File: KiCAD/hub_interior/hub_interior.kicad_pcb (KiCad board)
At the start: 2 copper layers, 50 x 50 mm, 15 parts, among them Q1 BC337, X2 BUZZER, X3 LED_ROJO

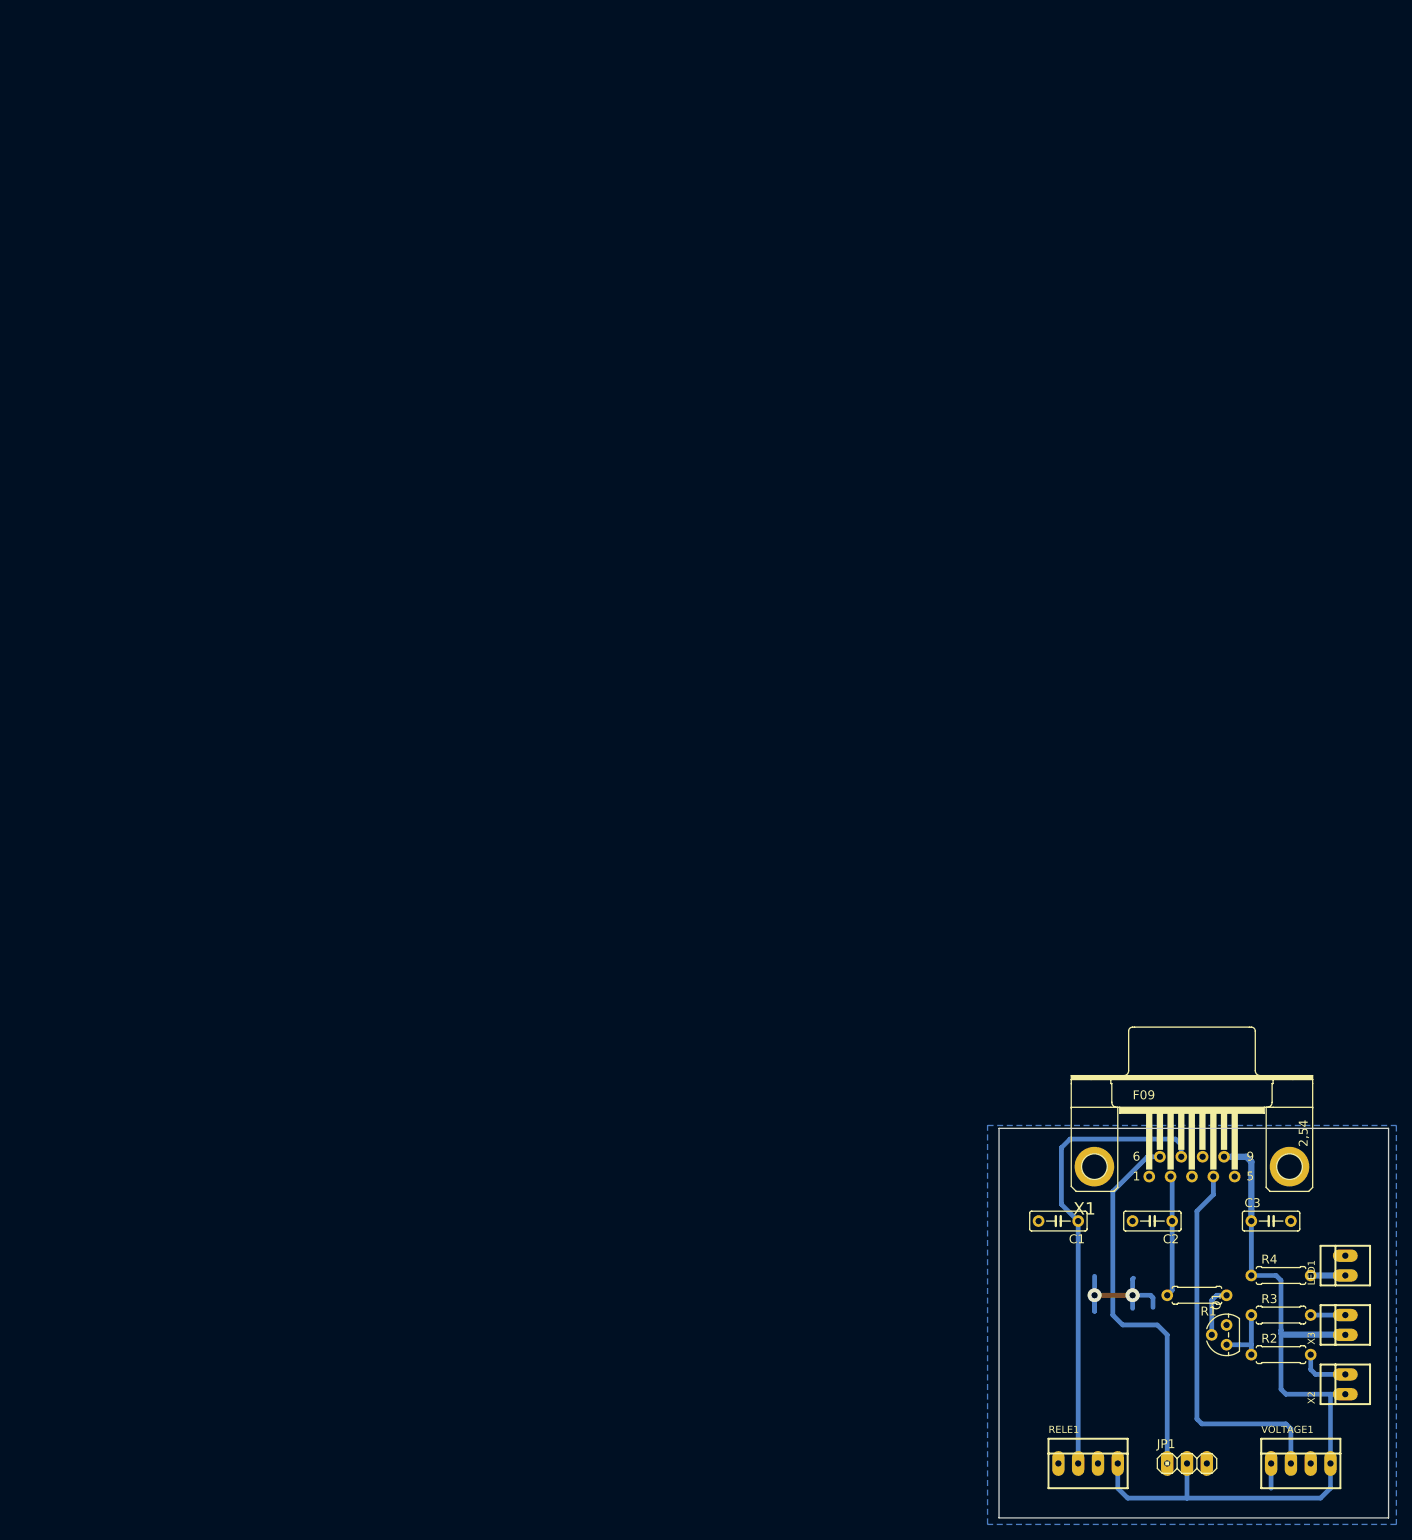
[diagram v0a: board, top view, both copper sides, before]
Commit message: rediseño hub interior
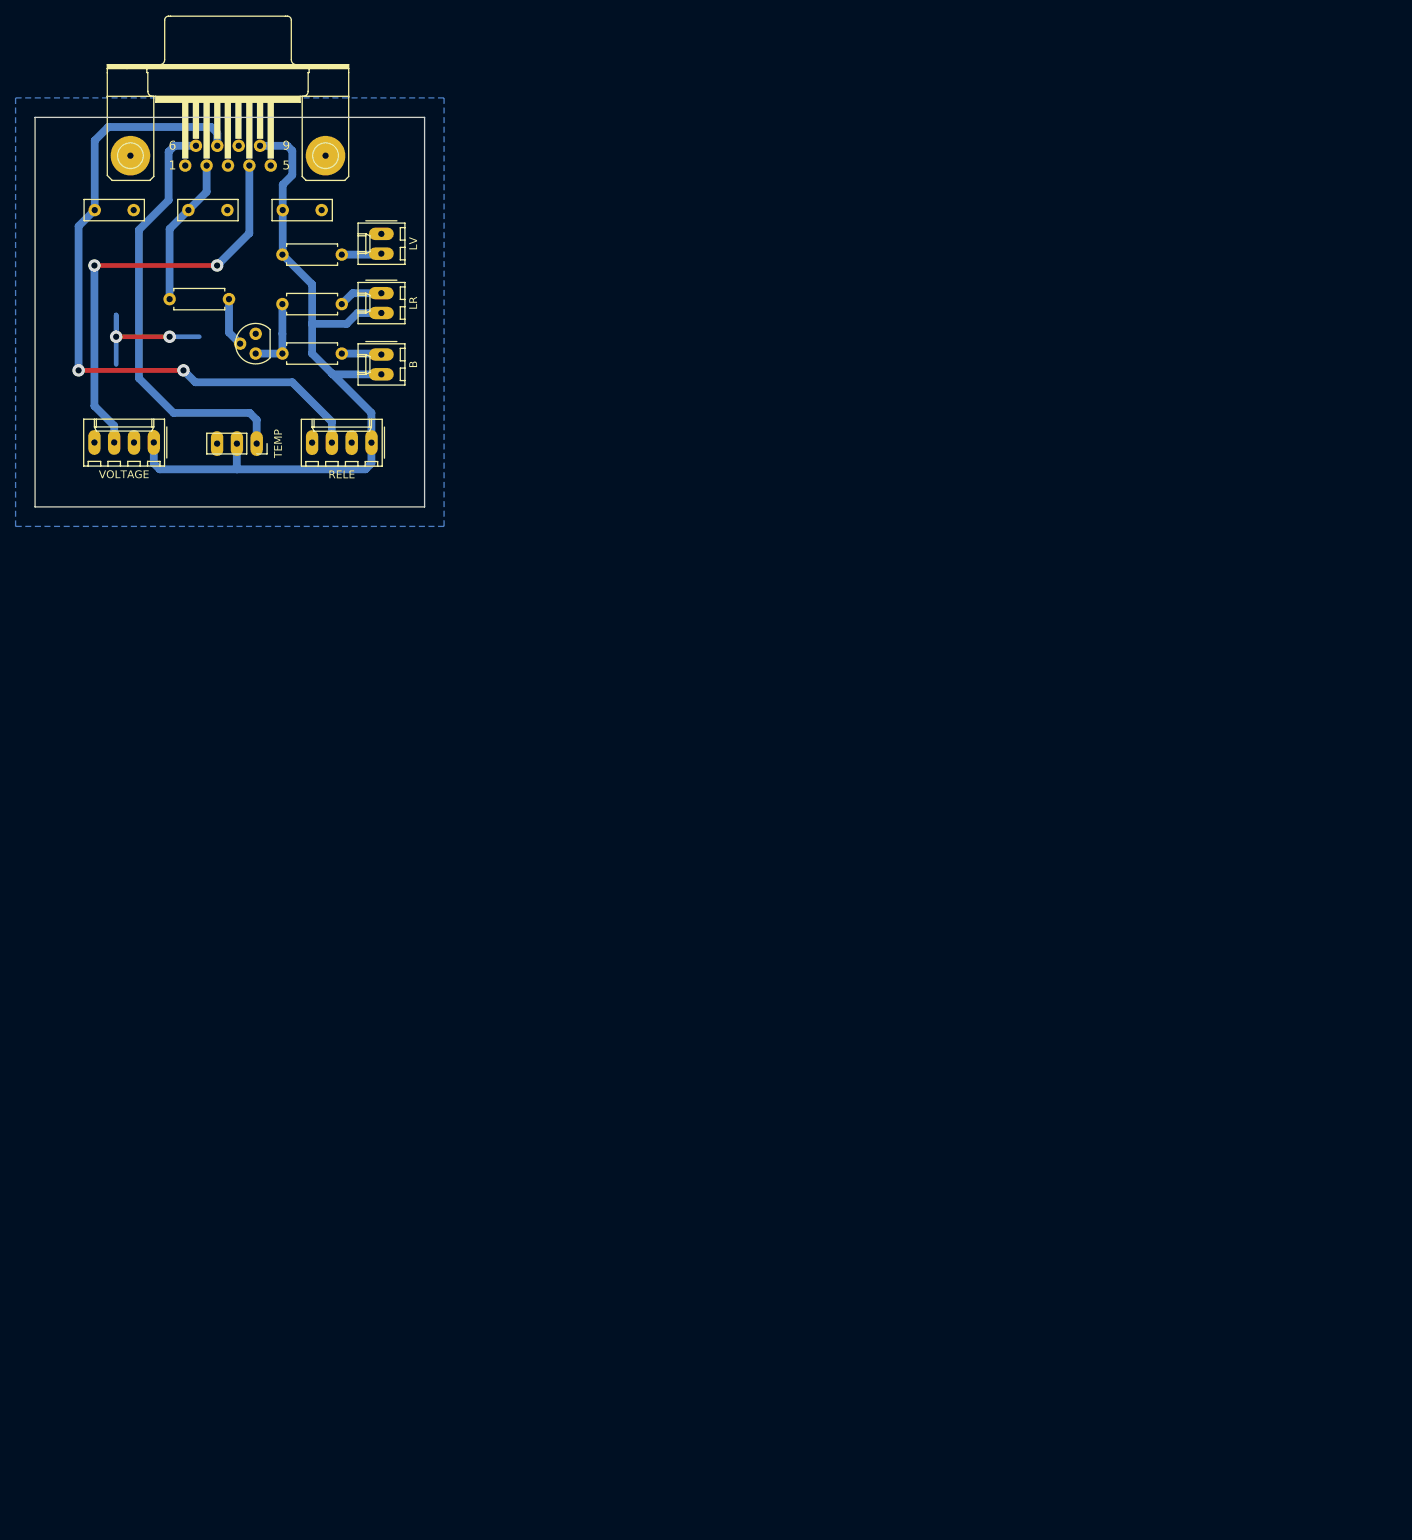
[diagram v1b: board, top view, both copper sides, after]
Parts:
- removed C3: 10nF, hub_interior:C050-025X075
- removed JP1: , hub_interior:1X03
- removed LED1: LED_VERDE, hub_interior:22-23-2021
- removed RELE1, VOLTAGE1: 22-23-2041, hub_interior:22-23-2041
- removed X2: BUZZER, hub_interior:22-23-2021
- removed X3: LED_ROJO, hub_interior:22-23-2021
- added B: BUZZER, Connector_Molex:Molex_KK-254_AE-6410-02A_1x02_P2.54mm_Vertical, F.Cu at (44.5, -19.6)
- added C4: 10nF, Capacitor_THT:C_Disc_D7.5mm_W2.5mm_P5.00mm, F.Cu at (7.66, -38.1)
- added LR: LED_ROJO, Connector_Molex:Molex_KK-254_AE-6410-02A_1x02_P2.54mm_Vertical, F.Cu at (44.5, -27.4)
- added LV: LED_VERDE, Connector_Molex:Molex_KK-254_AE-6410-02A_1x02_P2.54mm_Vertical, F.Cu at (44.5, -35.1)
- added RELE: 22-23-2041, Connector_Molex:Molex_KK-254_AE-6410-04A_1x04_P2.54mm_Vertical, F.Cu at (43.2, -8.26)
- added TEMP: PINHD-1X3, Connector_PinSocket_2.54mm:PinSocket_1x03_P2.54mm_Vertical, F.Cu at (28.4, -8.13)
- added VOLTAGE: 22-23-2041, Connector_Molex:Molex_KK-254_AE-6410-04A_1x04_P2.54mm_Vertical, F.Cu at (15.2, -8.28)
- C1: value (none) -> 10nF; footprint hub_interior:C050-025X075 -> Capacitor_THT:C_Disc_D7.5mm_W2.5mm_P5.00mm
- C2: footprint hub_interior:C050-025X075 -> Capacitor_THT:C_Disc_D7.5mm_W2.5mm_P5.00mm
- Q1: footprint hub_interior:TO92 -> Package_TO_SOT_THT:TO-92
- R1, R2, R3, R4: footprint hub_interior:0207_7 -> Resistor_THT:R_Axial_DIN0207_L6.3mm_D2.5mm_P7.62mm_Horizontal
- X1: value (none) -> F09HP
- moved R4 183.3 mm to (31.8, -32.4)
- moved R3 182.4 mm to (31.8, -26.0)
- moved R2 181.5 mm to (31.8, -19.7)
- moved X1 179.3 mm to (24.8, -45.1)
- moved R1 178.3 mm to (24.9, -26.7)
- moved Q1 177.2 mm to (28.3, -19.7)
- moved C1 171.2 mm to (19.7, -38.1), turned to 0 degrees
- moved C2 171.2 mm to (31.8, -38.1), turned to 0 degrees
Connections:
- C1 pad 1: N$4 -> Net-(C1-Pad1)
- C2 pad 1: N$2 -> +5V
- R1 pad 2: N$2 -> Net-(C1-Pad1)
- X1 pad 1: (no net) -> unconnected-(X1-Pad1)
- X1 pad 2: N$2 -> Net-(C1-Pad1)
- X1 pad 3: (no net) -> unconnected-(X1-Pad3)
- X1 pad 5: (no net) -> unconnected-(X1-Pad5)
- X1 pad 7: N$4 -> Net-(C4-Pad1)
- X1 pad 8: (no net) -> unconnected-(X1-Pad8)
- X1 pad G1: GND -> unconnected-(X1-PadG1)
- X1 pad G2: GND -> unconnected-(X1-PadG2)
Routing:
- net Net-(C4-Pad1): track 0.00 -> 86.7 mm, vias 0 -> 2
- net N$4: track 59.1 -> 0.00 mm
- net Net-(C1-Pad1): track 0.00 -> 19.1 mm
- net N$2: track 15.6 -> 0.00 mm
- net Net-(JP1-Pad1): track 48.3 -> 54.9 mm
- net Net-(VOLTAGE0-Pad2): track 49.0 -> 54.1 mm, vias 0 -> 2
- net GND: track 22.8 -> 19.8 mm
- net +5V: track 101.8 -> 100.2 mm
- net Net-(Q1-Pad3): track 8.26 -> 9.78 mm
- net Net-(R2-Pad2): track 6.61 -> 5.13 mm
- net Net-(R3-Pad2): track 4.45 -> 5.66 mm
- net Net-(Q1-Pad2): track 6.61 -> 5.67 mm
- net Net-(LED0-Pad1): track 4.45 -> 5.13 mm
